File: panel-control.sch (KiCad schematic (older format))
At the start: 60 parts, among them J1 POWER_CONN, J2 SWIM, J3 PWR, J4 40HAT, J5 HUB-75_A, J6 HUB-75_B, J7 VBAT, J8 FAN, J9 MK_R, Q1 DMMT5401, Q2 DMG2305UX, Q3 AO4407A, Q4 S8050, SW1 POW, SW2 NRST, U1 TXS0108EPW, U2 TXS0108EPW, U3 TXS0108EPW, U4 HT7533-1, U5 STM8S103F3P

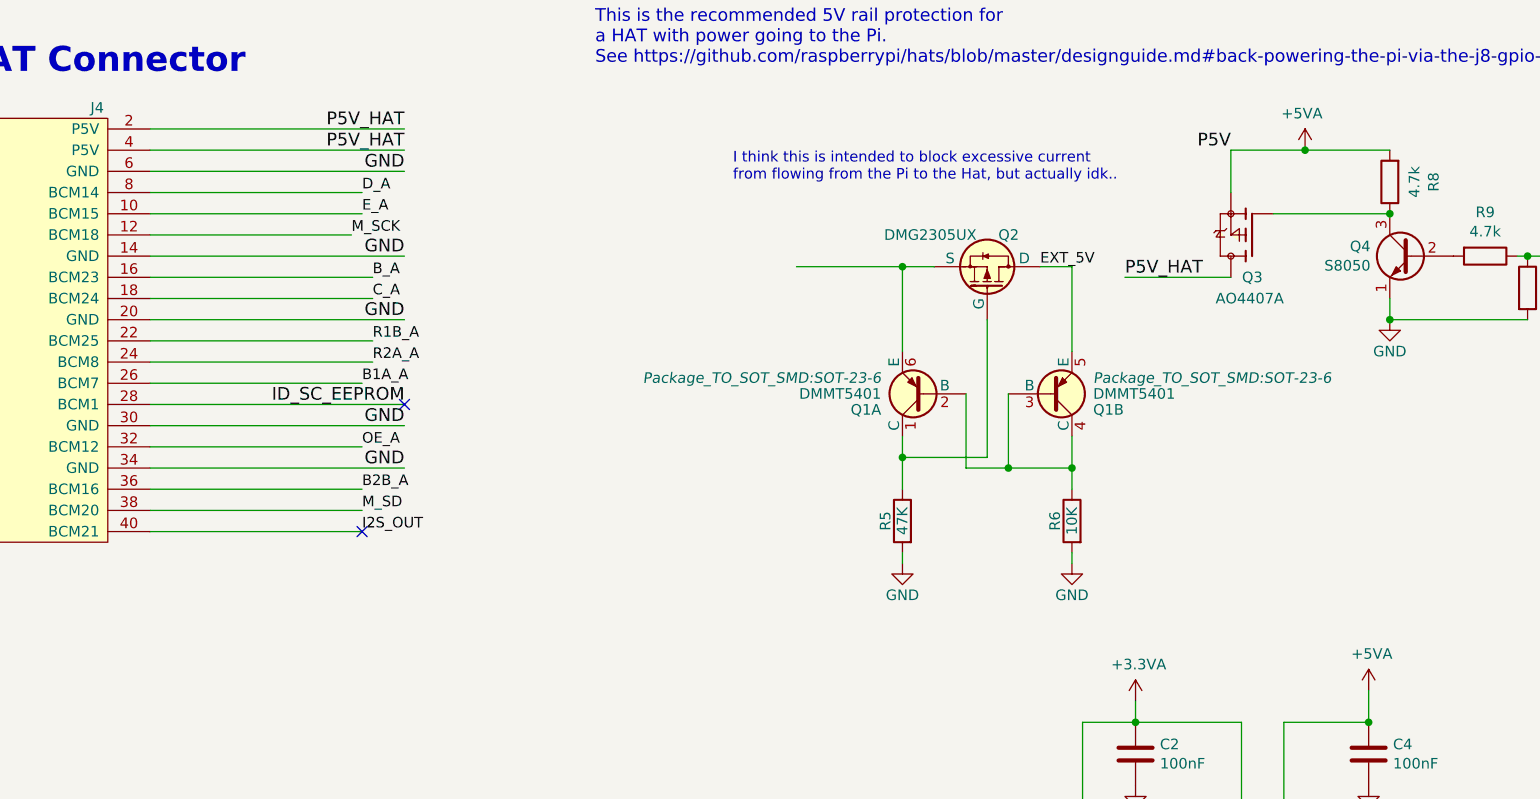
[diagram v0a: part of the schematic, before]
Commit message: nearly ready to submit
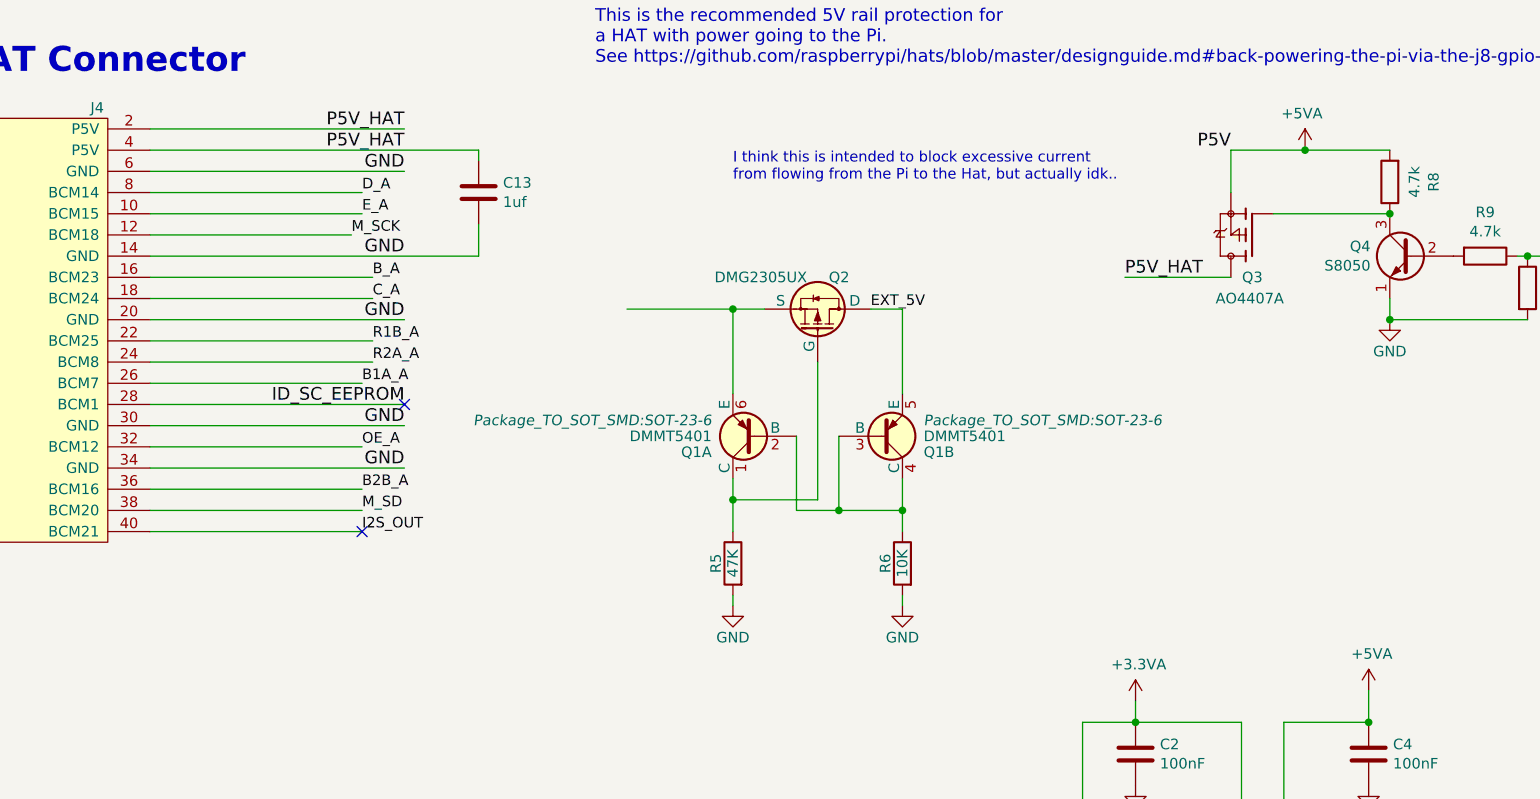
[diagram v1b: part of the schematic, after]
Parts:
- added C13: 1uf, Capacitor_SMD:C_1206_3216Metric, symbol Device:C
- J1: footprint Connector_PinHeader_2.54mm:PinHeader_1x06_P2.54mm_Vertical -> Connector_FFC-FPC:Molex_200528-0060_1x06-1MP_P1.00mm_Horizontal
- Q3: footprint SOIC127P600X175-8N -> libraries:SOIC127P600X175-8N
- R1, R10, R12, R13, R15, R16, R17, R18, R19, R2, R3, R4, R8, R9: footprint Resistor_SMD:R_0603_1608Metric -> Resistor_SMD:R_0402_1005Metric
- R11: footprint Resistor_SMD:R_0603_1608Metric_Pad0.98x0.95mm_HandSolder -> Resistor_SMD:R_0402_1005Metric
- R7: footprint Capacitor_SMD:C_0603_1608Metric_Pad1.08x0.95mm_HandSolder -> Capacitor_SMD:C_0402_1005Metric
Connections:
- wire segments 261 -> 263
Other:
- moved on the sheet: Q1A, Q1B, Q2, R5, R6
